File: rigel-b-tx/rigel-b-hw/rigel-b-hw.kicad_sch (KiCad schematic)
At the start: 57 parts, among them IC1 BALFHB-WL-02D3, J4 BCS-102-L-D-TE, J5 S2B-XH-A, U1 STM32WLE5C8Ux, U2 TPS629206DRLR, U3 CH340X, U4 TYPE-C_16PIN_2MD(073), U5 X1G004131004200, U6 KH-SMA-K513-G, U7 MSK12C02-HB, U8 SAM-M10Q-00B, U9 BGS12WN6E6327XTSA1

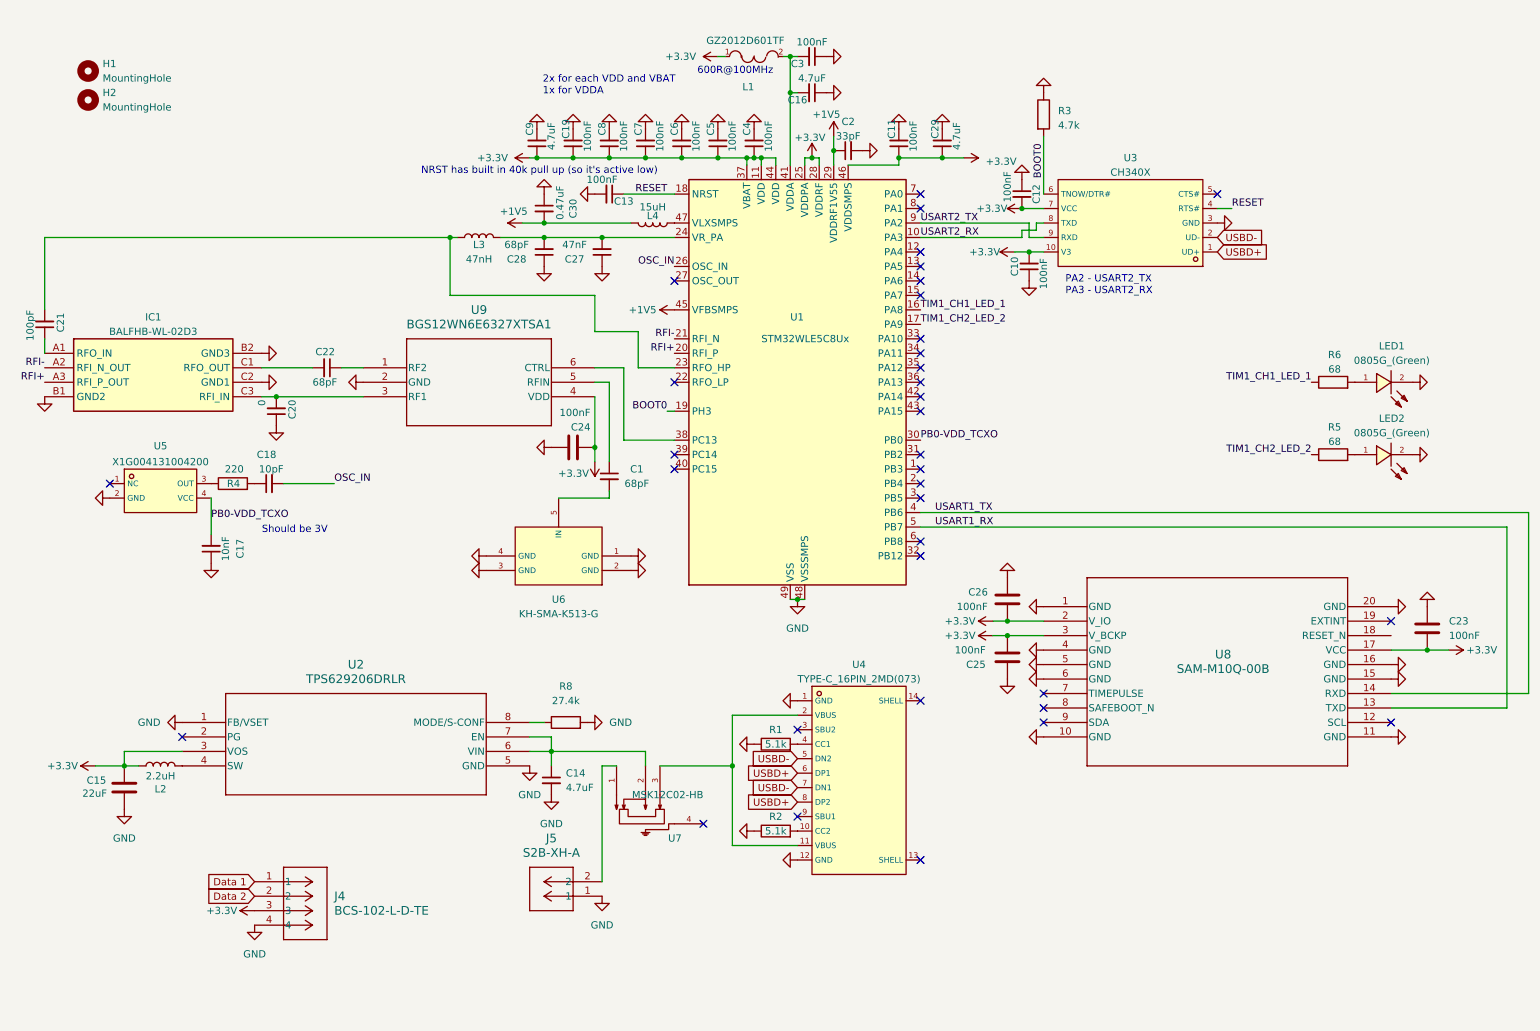
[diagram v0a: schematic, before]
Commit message: RF Switch finalized
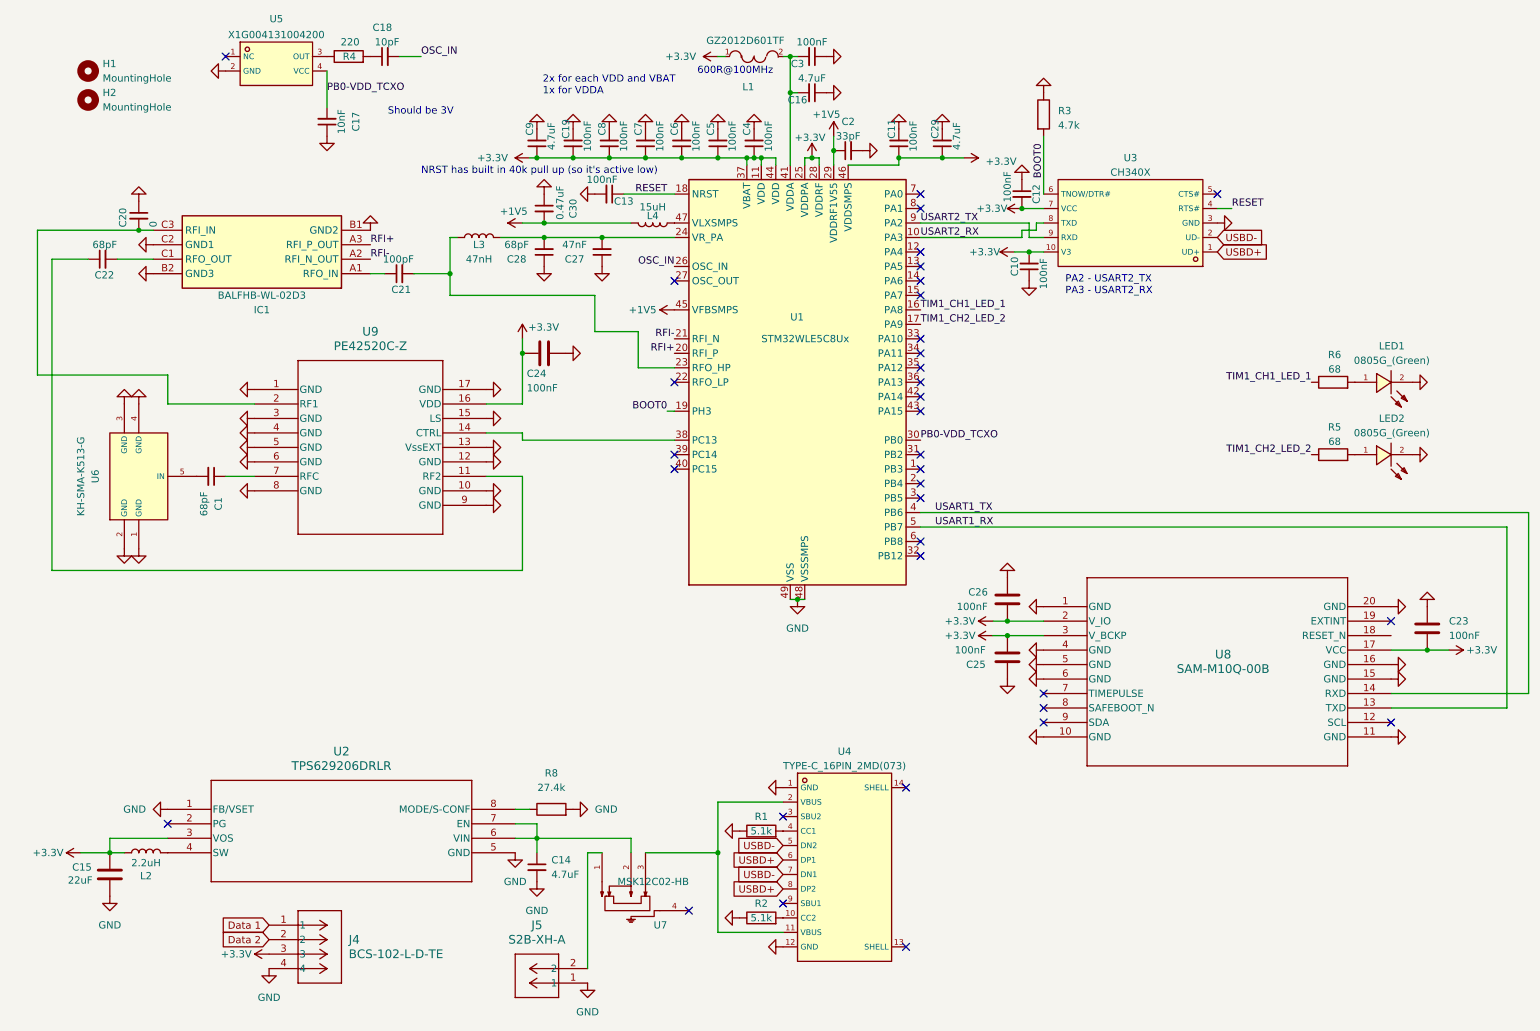
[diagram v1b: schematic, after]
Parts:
- removed U9: BGS12WN6E6327XTSA1, jlc:PG-TSNP-6-10_INF, symbol 2024-11-10_21-59-30:BGS12WN6E6327XTSA1
- added U9: PE42520C-Z, QFN_2520C-Z_PSM, symbol 2025-02-07_21-48-15:PE42520C-Z
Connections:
- net +3.3V: now also U9.16 (VDD)
- net GND: now also U9.1 (GND), U9.10 (GND), U9.12 (GND), U9.13 (VssEXT), U9.15 (LS), U9.17 (GND), U9.3 (GND), U9.4 (GND), U9.5 (GND), U9.6 (GND), U9.8 (GND), U9.9 (GND)
- net at C20.2, IC1.C3 (RFI_IN): now also U9.2 (RF1)
- net at C1.1: now also U9.7 (RFC)
- net at C22.1: now also U9.11 (RF2)
- net at U1.38 (PC13): now also U9.14 (CTRL)
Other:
- moved on the sheet: C1, C14, C15, C17, C18, C20, C21, C22, C24, IC1, J4, J5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
